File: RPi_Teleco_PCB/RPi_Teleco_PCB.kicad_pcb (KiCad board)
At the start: 2 copper layers, 116.8 x 81.3 mm, 18 parts, among them J1 Conn_01x07, M3 MountingHole_3.2mm_M3, Q1 PN2222A, U1 MCP23017_SP

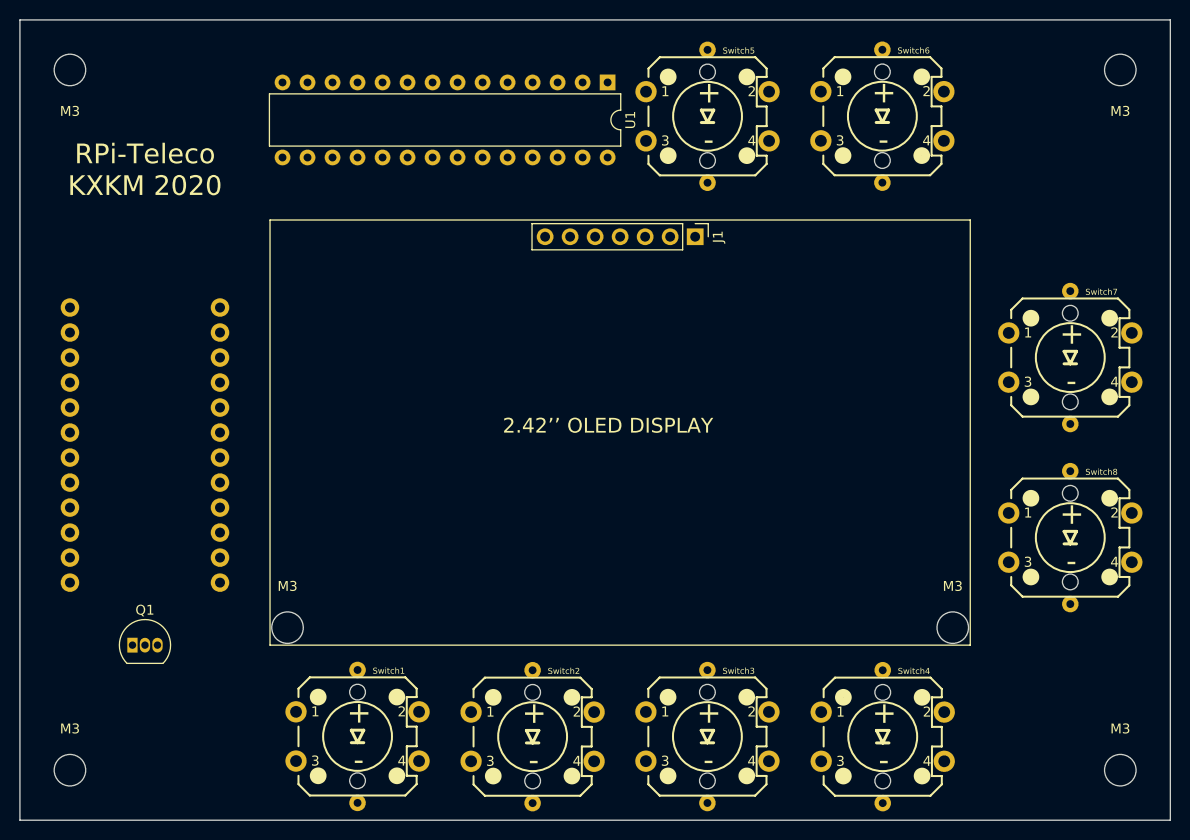
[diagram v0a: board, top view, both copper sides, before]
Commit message: ready
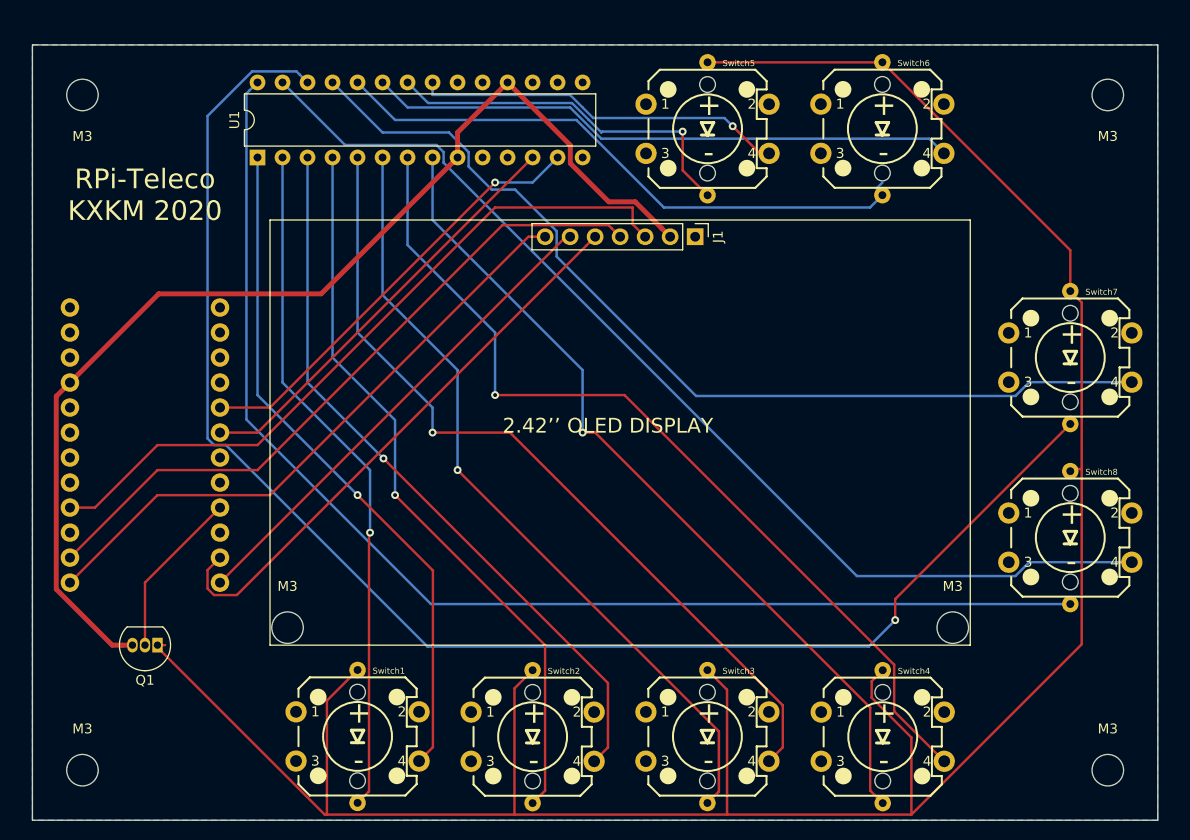
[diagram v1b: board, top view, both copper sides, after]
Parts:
- removed the M3 at (124.5, 48.3)
- removed the M3 at (231.1, 48.3)
- added M3: MountingHole_3.2mm_M3, MountingHole:MountingHole_3.2mm_M3, F.Cu at (125.7, 50.8)
- added M3: MountingHole_3.2mm_M3, MountingHole:MountingHole_3.2mm_M3, F.Cu at (229.9, 50.8)
- moved U1 36.4 mm to (143.5, 57.1), turned to 90 degrees
- moved Q1 2.54 mm to (133.3, 106.7), turned to 180 degrees
- moved M3 1.27 mm to (125.7, 119.4)
- moved Switch5 1.27 mm to (189.2, 54.2)
- moved Switch6 1.27 mm to (207.0, 54.2)
- moved M3 1.27 mm to (229.9, 119.4)
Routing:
- net Level: track 0.00 -> 259.4 mm
- net LED7: track 0.00 -> 152.3 mm, vias 0 -> 1
- net LED8: track 0.00 -> 126.1 mm
- net +5V: track 0.00 -> 115.1 mm
- net BTN8: track 0.00 -> 108.2 mm
- net BTN7: track 0.00 -> 97.3 mm
- net BTN4: track 0.00 -> 91.6 mm, vias 0 -> 1
- net LED4: track 0.00 -> 85.3 mm, vias 0 -> 1
- net BTN3: track 0.00 -> 84.4 mm, vias 0 -> 1
- net LED3: track 0.00 -> 80.2 mm, vias 0 -> 1
- net LED2: track 0.00 -> 75.0 mm, vias 0 -> 1
- net BTN2: track 0.00 -> 74.5 mm, vias 0 -> 1
- net SCK: track 0.00 -> 73.3 mm
- net SDA: track 0.00 -> 70.4 mm
- net LED1: track 0.00 -> 69.8 mm, vias 0 -> 1
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- added copper zone on B.Cu, net GND
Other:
- board size 116.8 x 81.3 mm -> 114.3 x 78.7 mm
